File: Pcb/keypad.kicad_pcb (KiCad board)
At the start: 2 copper layers, 66 x 85 mm, 5 parts, among them SW1 SW_Push, SW2 SW_Push, SW3 SW_Push, SW4 SW_Push, U1 MOUDLE-SEEEDUINO-XIAO

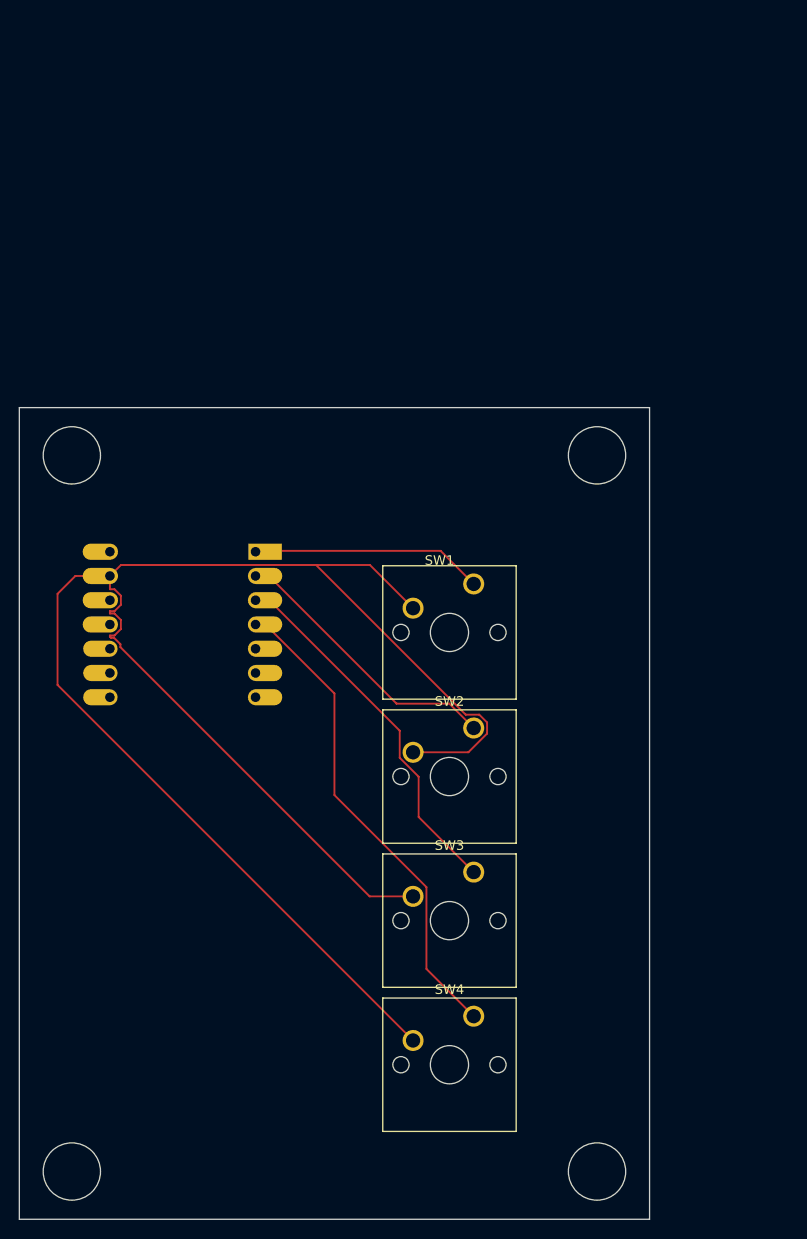
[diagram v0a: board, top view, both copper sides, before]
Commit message: fixed base design
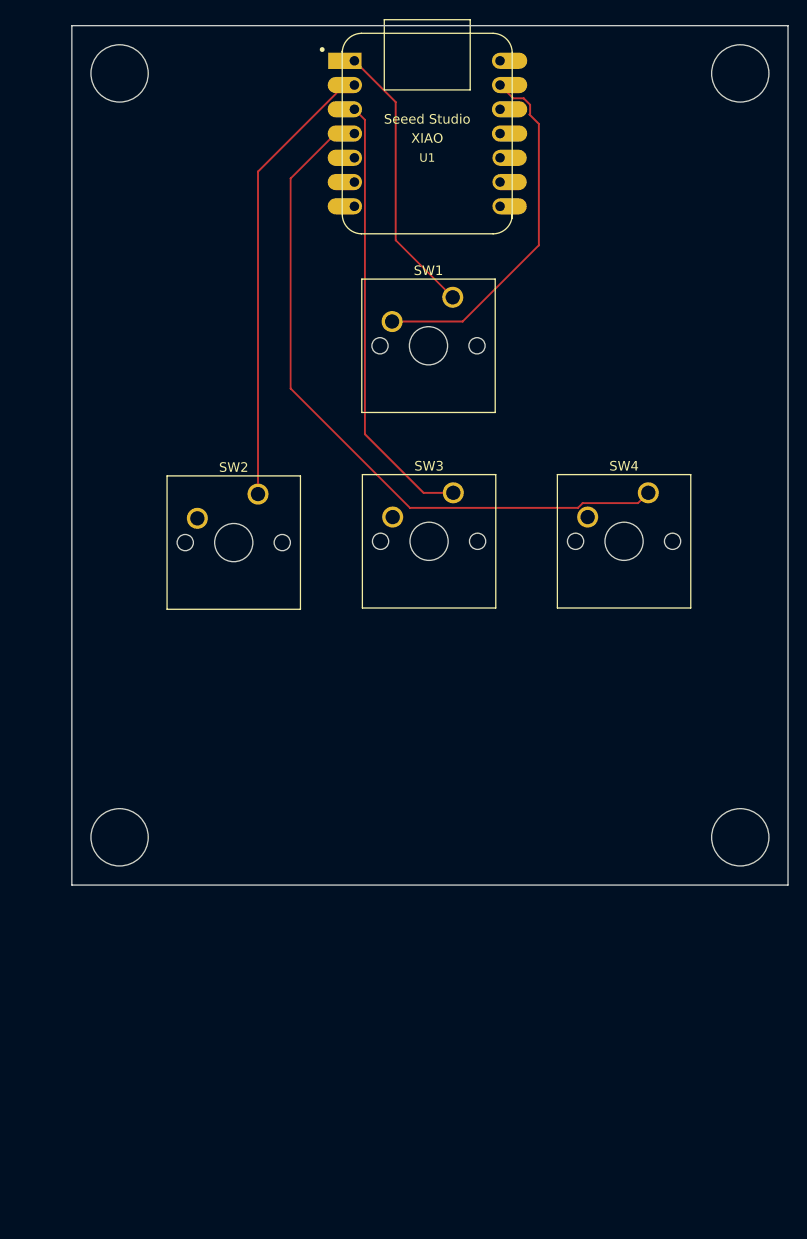
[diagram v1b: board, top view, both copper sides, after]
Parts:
- U1: moved to F.Cu
- moved SW4 57.8 mm to (170.4, 68.9)
- moved U1 57.4 mm to (147.2, 31.3), turned to 0 degrees
- moved SW3 39.8 mm to (149.9, 68.9)
- moved SW2 33.3 mm to (129.5, 69.1)
- moved SW1 30.1 mm to (149.9, 48.4)
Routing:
- net GND: track 210.0 -> 37.8 mm
- net Net-(U1-PA11_A3_D3): track 51.1 -> 73.9 mm
- net Net-(U1-PA4_A1_D1): track 29.4 -> 47.6 mm
- net Net-(U1-PA10_A2_D2): track 38.8 -> 46.3 mm
- net Net-(U1-PA02_A0_D0): track 24.3 -> 29.0 mm
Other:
- board size 66 x 85 mm -> 75 x 90 mm
